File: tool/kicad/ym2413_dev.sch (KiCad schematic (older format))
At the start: 146 parts, among them J1 MICRO-USB-AB, K1 CONN_3, K2 CONN_3, P1 TEST_POINT, P10 TEST_POINT, P11 TEST_POINT, P12 TEST_POINT, P13 TEST_POINT, P14 TEST_POINT, P15 TEST_POINT, P16 TEST_POINT, P17 TEST_POINT, P18 TEST_POINT, P19 TEST_POINT, P2 TEST_POINT, P20 TEST_POINT, P21 TEST_POINT, P22 TEST_POINT, P23 TEST_POINT, P24 TEST_POINT, P25 TEST_POINT, P26 TEST_POINT, P27 TEST_POINT, P28 TEST_POINT, P29 TEST_POINT, P3 TEST_POINT, P30 CONN_3X2, P31 CONN_2, P32 CONN_2, P33 TEST_POINT, P34 TEST_POINT, P35 CONN_6, P37 TEST_POINT, P38 TEST_POINT, P4 TEST_POINT, P5 MIDI-IN, P6 TEST_POINT, P7 TEST_POINT, P8 TEST_POINT, P9 TEST_POINT, U1 SN74LVC2T45, U2 ST-USBLC6-2, U3 EFM32GG332, U4 YM2413, U5 LM386, U6 LM386, U7 ACPL-M21L, X1 48Mhz, X2 CRYSTAL

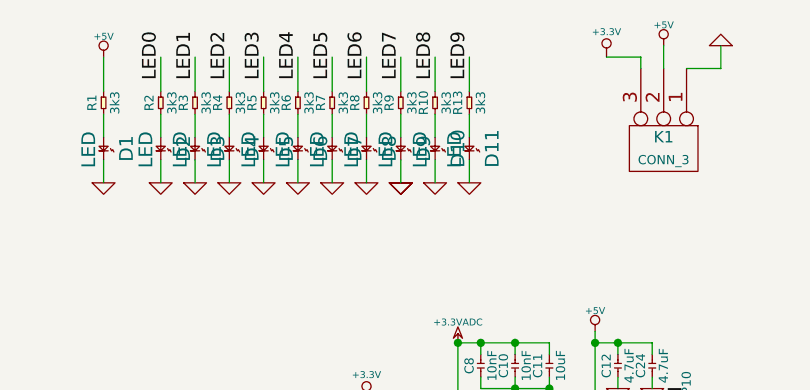
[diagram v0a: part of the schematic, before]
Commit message: finish first layout
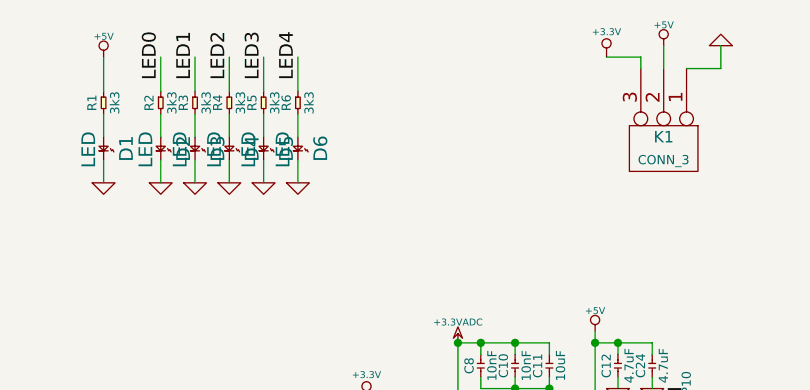
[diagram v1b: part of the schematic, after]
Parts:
- removed D10, D11, D7, D8, D9: LED, symbol LED
- removed R10, R13, R7, R8, R9: 3k3, symbol R
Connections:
- wire segments 360 -> 345
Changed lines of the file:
@@
 	2750 1250 2750 1400
-$Comp
-L R R7
-U 1 1 52F7EF20
-P 2900 1450
-F 0 "R7" H 2900 1500 40  0000 C CNN
-F 1 "3k3" H 2900 1400 40  0000 C CNN
-F 2 "" H 2900 1450 60  0000 C CNN
-F 3 "" H 2900 1450 60  0000 C CNN
-	1    2900 1450
-	0    -1   -1   0
-$EndComp
-$Comp
-L LED D7
-U 1 1 52F7EF26
-P 2900 1650
-F 0 "D7" H 2900 1750 60  0000 C CNN
-F 1 "LED" H 2905 1585 60  0000 C CNN
-F 2 "" H 2900 1650 60  0000 C CNN
-F 3 "" H 2900 1650 60  0000 C CNN
-	1    2900 1650
-	0    1    1    0
-$EndComp
-Wire Wire Line
-	2900 1500 2900 1600
-Wire Wire Line
-	2900 1800 2900 1700
-$Comp
-L GND #PWR043
-U 1 1 52F7EF2E
-P 2900 1800
-F 0 "#PWR043" H 2900 1800 30  0001 C CNN
-F 1 "GND" H 2900 1730 30  0001 C CNN
-F 2 "" H 2900 1800 60  0000 C CNN
-F 3 "" H 2900 1800 60  0000 C CNN
-	1    2900 1800
-	1    0    0    -1
-$EndComp
-Wire Wire Line
-	2900 1250 2900 1400
-$Comp
-L R R8
-U 1 1 52F7EF35
-P 3050 1450
-F 0 "R8" H 3050 1500 40  0000 C CNN
-F 1 "3k3" H 3050 1400 40  0000 C CNN
-F 2 "" H 3050 1450 60  0000 C CNN
-F 3 "" H 3050 1450 60  0000 C CNN
-	1    3050 1450
-	0    -1   -1   0
-$EndComp
-$Comp
-L LED D8
-U 1 1 52F7EF3B
-P 3050 1650
-F 0 "D8" H 3050 1750 60  0000 C CNN
-F 1 "LED" H 3055 1585 60  0000 C CNN
-F 2 "" H 3050 1650 60  0000 C CNN
-F 3 "" H 3050 1650 60  0000 C CNN
-	1    3050 1650
-	0    1    1    0
-$EndComp
-Wire Wire Line
-	3050 1500 3050 1600
-Wire Wire Line
-	3050 1800 3050 1700
-$Comp
-L GND #PWR044
-U 1 1 52F7EF43
-P 3050 1800
-F 0 "#PWR044" H 3050 1800 30  0001 C CNN
-F 1 "GND" H 3050 1730 30  0001 C CNN
-F 2 "" H 3050 1800 60  0000 C CNN
-F 3 "" H 3050 1800 60  0000 C CNN
-	1    3050 1800
-	1    0    0    -1
-$EndComp
-Wire Wire Line
-	3050 1250 3050 1400
-$Comp
-L R R9
-U 1 1 52F7EF4A
-P 3200 1450
-F 0 "R9" H 3200 1500 40  0000 C CNN
-F 1 "3k3" H 3200 1400 40  0000 C CNN
-F 2 "" H 3200 1450 60  0000 C CNN
-F 3 "" H 3200 1450 60  0000 C CNN
-	1    3200 1450
-	0    -1   -1   0
-$EndComp
-$Comp
-L LED D9
-U 1 1 52F7EF50
-P 3200 1650
-F 0 "D9" H 3200 1750 60  0000 C CNN
-F 1 "LED" H 3205 1585 60  0000 C CNN
-F 2 "" H 3200 1650 60  0000 C CNN
-F 3 "" H 3200 1650 60  0000 C CNN
-	1    3200 1650
-	0    1    1    0
-$EndComp
-Wire Wire Line
-	3200 1500 3200 1600
-Wire Wire Line
-	3200 1800 3200 1700
-$Comp
-L GND #PWR045
-U 1 1 52F7EF58
-P 3200 1800
-F 0 "#PWR045" H 3200 1800 30  0001 C CNN
-F 1 "GND" H 3200 1730 30  0001 C CNN
-F 2 "" H 3200 1800 60  0000 C CNN
-F 3 "" H 3200 1800 60  0000 C CNN
-	1    3200 1800
-	1    0    0    -1
-$EndComp
-Wire Wire Line
-	3200 1250 3200 1400
-$Comp
-L GND #PWR046
-U 1 1 52F7EF5F
-P 3200 1800
-F 0 "#PWR046" H 3200 1800 30  0001 C CNN
-F 1 "GND" H 3200 1730 30  0001 C CNN
-F 2 "" H 3200 1800 60  0000 C CNN
-F 3 "" H 3200 1800 60  0000 C CNN
-	1    3200 1800
-	1    0    0    -1
-$EndComp
-$Comp
-L R R10
-U 1 1 52F7EF65
-P 3350 1450
-F 0 "R10" H 3350 1500 40  0000 C CNN
-F 1 "3k3" H 3350 1400 40  0000 C CNN
-F 2 "" H 3350 1450 60  0000 C CNN
-F 3 "" H 3350 1450 60  0000 C CNN
-	1    3350 1450
-	0    -1   -1   0
-$EndComp
-$Comp
-L LED D10
-U 1 1 52F7EF6B
-P 3350 1650
-F 0 "D10" H 3350 1750 60  0000 C CNN
-F 1 "LED" H 3355 1585 60  0000 C CNN
-F 2 "" H 3350 1650 60  0000 C CNN
-F 3 "" H 3350 1650 60  0000 C CNN
-	1    3350 1650
-	0    1    1    0
-$EndComp
-Wire Wire Line
-	3350 1500 3350 1600
-Wire Wire Line
-	3350 1800 3350 1700
-$Comp
-L GND #PWR047
-U 1 1 52F7EF73
-P 3350 1800
-F 0 "#PWR047" H 3350 1800 30  0001 C CNN
-F 1 "GND" H 3350 1730 30  0001 C CNN
-F 2 "" H 3350 1800 60  0000 C CNN
-F 3 "" H 3350 1800 60  0000 C CNN
-	1    3350 1800
-	1    0    0    -1
-$EndComp
-Wire Wire Line
-	3350 1250 3350 1400
-$Comp
-L R R13
-U 1 1 52F7EF7A
-P 3500 1450
-F 0 "R13" H 3500 1500 40  0000 C CNN
-F 1 "3k3" H 3500 1400 40  0000 C CNN
-F 2 "" H 3500 1450 60  0000 C CNN
-F 3 "" H 3500 1450 60  0000 C CNN
-	1    3500 1450
-	0    -1   -1   0
-$EndComp
-$Comp
-L LED D11
-U 1 1 52F7EF80
-P 3500 1650
-F 0 "D11" H 3500 1750 60  0000 C CNN
-F 1 "LED" H 3505 1585 60  0000 C CNN
-F 2 "" H 3500 1650 60  0000 C CNN
-F 3 "" H 3500 1650 60  0000 C CNN
-	1    3500 1650
-	0    1    1    0
-$EndComp
-Wire Wire Line
-	3500 1500 3500 1600
-Wire Wire Line
-	3500 1800 3500 1700
-$Comp
-L GND #PWR048
-U 1 1 52F7EF88
-P 3500 1800
-F 0 "#PWR048" H 3500 1800 30  0001 C CNN
-F 1 "GND" H 3500 1730 30  0001 C CNN
-F 2 "" H 3500 1800 60  0000 C CNN
-F 3 "" H 3500 1800 60  0000 C CNN
-	1    3500 1800
-	1    0    0    -1
-$EndComp
-Wire Wire Line
-	3500 1250 3500 1400
 $Comp
 L +5V #PWR049
@@
 Text Label 2750 1350 1    60   ~ 0
 LED4
-Text Label 2900 1350 1    60   ~ 0
-LED5
-Text Label 3050 1350 1    60   ~ 0
-LED6
-Text Label 3200 1350 1    60   ~ 0
-LED7
-Text Label 3350 1350 1    60   ~ 0
-LED8
-Text Label 3500 1350 1    60   ~ 0
-LED9
 Wire Wire Line
 	4900 5750 4900 5600
